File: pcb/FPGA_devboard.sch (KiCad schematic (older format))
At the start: 2 parts, among them X5 Conn_02x06_Odd_Even, X6 AC7020

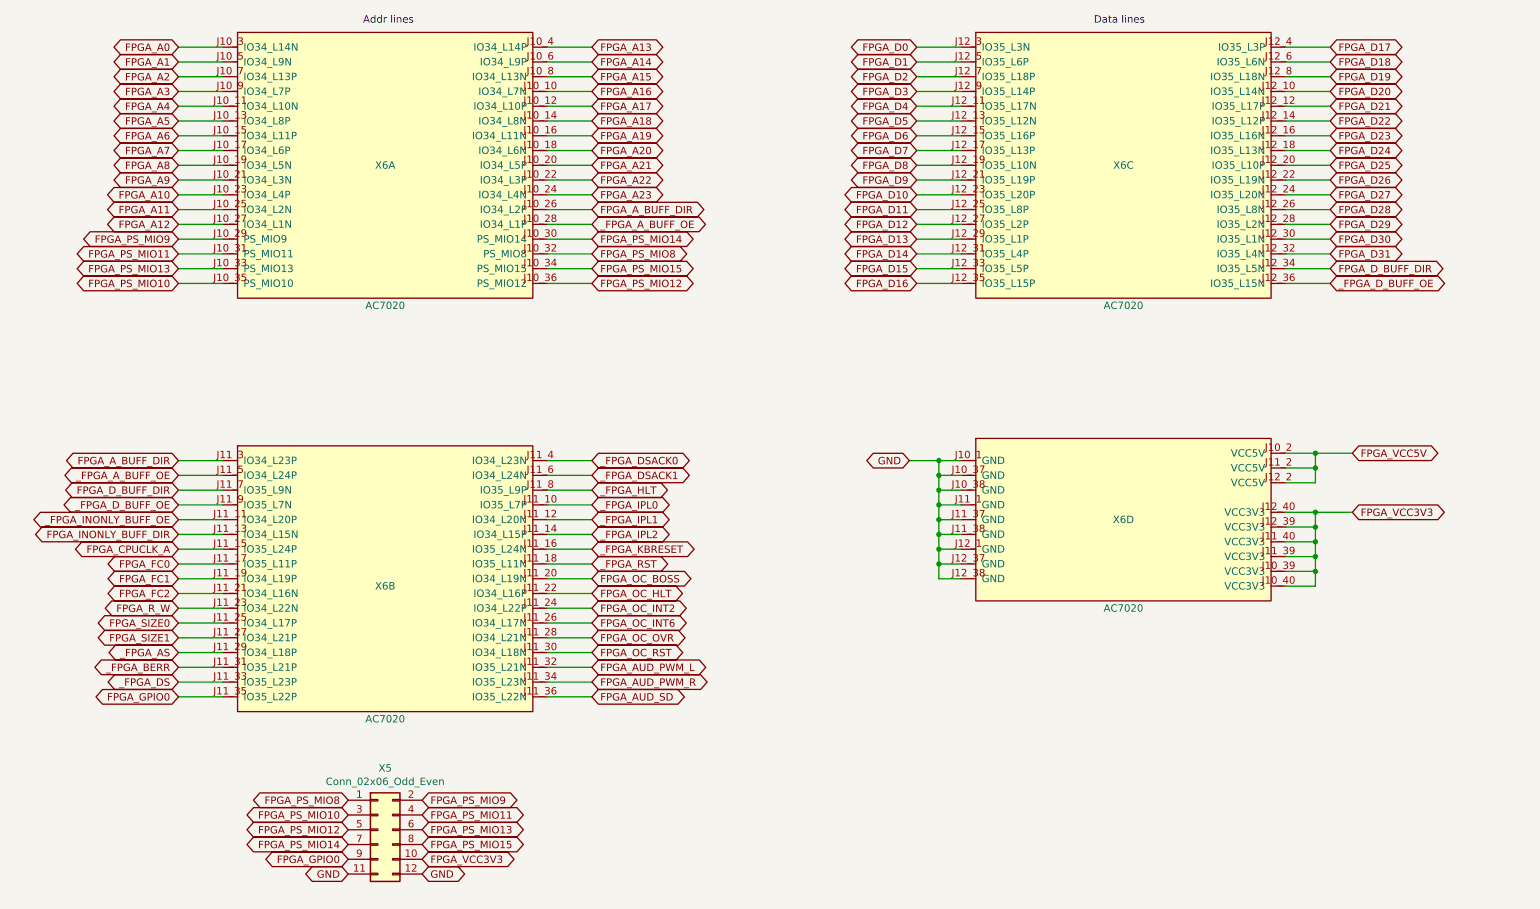
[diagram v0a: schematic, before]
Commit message: Some more changes wip
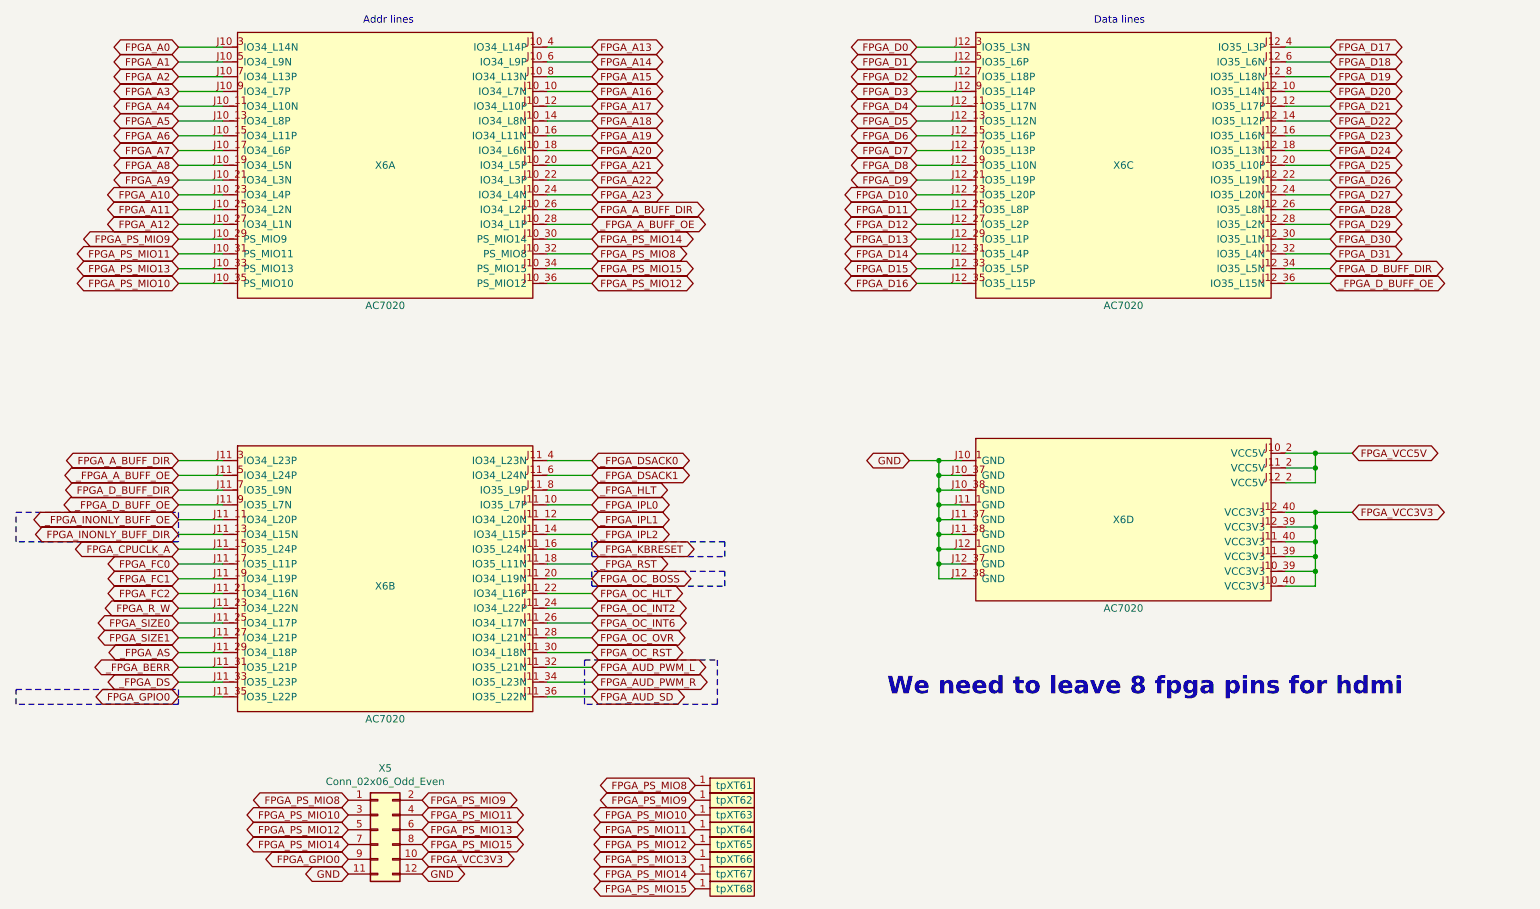
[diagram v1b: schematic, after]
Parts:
- added XT61, XT62, XT63, XT64, XT65, XT66, XT67, XT68: testpoint, symbol WM1200:testpoint
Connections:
- net FPGA_PS_MIO10: now also XT63.1 (tp)
- net FPGA_PS_MIO11: now also XT64.1 (tp)
- net FPGA_PS_MIO12: now also XT65.1 (tp)
- net FPGA_PS_MIO13: now also XT66.1 (tp)
- net FPGA_PS_MIO14: now also XT67.1 (tp)
- net FPGA_PS_MIO15: now also XT68.1 (tp)
- net FPGA_PS_MIO8: now also XT61.1 (tp)
- net FPGA_PS_MIO9: now also XT62.1 (tp)
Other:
- note added: "We need to leave 8 fpga pins for hdmi"
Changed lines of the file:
@@
 Wire Wire Line
 	4600 3200 4300 3200
+$Comp
+L WM1200:testpoint XT61
+U 1 1 5E5A11BD
+P 5550 6650
+F 0 "XT61" H 5600 6700 50  0000 C CNN
+F 1 "testpoint" H 5550 6800 50  0001 C CNN
+F 2 "" H 5550 6650 50  0001 C CNN
+F 3 "" H 5550 6650 50  0001 C CNN
+	1    5550 6650
+	1    0    0    -1
+$EndComp
+$Comp
+L WM1200:testpoint XT62
+U 1 1 5E5B690A
+P 5550 6750
+F 0 "XT62" H 5600 6800 50  0000 C CNN
+F 1 "testpoint" H 5550 6900 50  0001 C CNN
+F 2 "" H 5550 6750 50  0001 C CNN
+F 3 "" H 5550 6750 50  0001 C CNN
+	1    5550 6750
+	1    0    0    -1
+$EndComp
+$Comp
+L WM1200:testpoint XT63
+U 1 1 5E5BE856
+P 5550 6850
+F 0 "XT63" H 5600 6900 50  0000 C CNN
+F 1 "testpoint" H 5550 7000 50  0001 C CNN
+F 2 "" H 5550 6850 50  0001 C CNN
+F 3 "" H 5550 6850 50  0001 C CNN
+	1    5550 6850
+	1    0    0    -1
+$EndComp
+$Comp
+L WM1200:testpoint XT64
+U 1 1 5E5C67D2
+P 5550 6950
+F 0 "XT64" H 5600 7000 50  0000 C CNN
+F 1 "testpoint" H 5550 7100 50  0001 C CNN
+F 2 "" H 5550 6950 50  0001 C CNN
+F 3 "" H 5550 6950 50  0001 C CNN
+	1    5550 6950
+	1    0    0    -1
+$EndComp
+$Comp
+L WM1200:testpoint XT65
+U 1 1 5E5CE745
+P 5550 7050
+F 0 "XT65" H 5600 7100 50  0000 C CNN
+F 1 "testpoint" H 5550 7200 50  0001 C CNN
+F 2 "" H 5550 7050 50  0001 C CNN
+F 3 "" H 5550 7050 50  0001 C CNN
+	1    5550 7050
+	1    0    0    -1
+$EndComp
+$Comp
+L WM1200:testpoint XT66
+U 1 1 5E5D6657
+P 5550 7150
+F 0 "XT66" H 5600 7200 50  0000 C CNN
+F 1 "testpoint" H 5550 7300 50  0001 C CNN
+F 2 "" H 5550 7150 50  0001 C CNN
+F 3 "" H 5550 7150 50  0001 C CNN
+	1    5550 7150
+	1    0    0    -1
+$EndComp
+$Comp
+L WM1200:testpoint XT67
+U 1 1 5E5DE64C
+P 5550 7250
+F 0 "XT67" H 5600 7300 50  0000 C CNN
+F 1 "testpoint" H 5550 7400 50  0001 C CNN
+F 2 "" H 5550 7250 50  0001 C CNN
+F 3 "" H 5550 7250 50  0001 C CNN
+	1    5550 7250
+	1    0    0    -1
+$EndComp
+$Comp
+L WM1200:testpoint XT68
+U 1 1 5E5E66B0
+P 5550 7350
+F 0 "XT68" H 5600 7400 50  0000 C CNN
+F 1 "testpoint" H 5550 7500 50  0001 C CNN
+F 2 "" H 5550 7350 50  0001 C CNN
+F 3 "" H 5550 7350 50  0001 C CNN
+	1    5550 7350
+	1    0    0    -1
+$EndComp
+Text GLabel 5300 6600 0    50   BiDi ~ 0
+FPGA_PS_MIO8
+Text GLabel 5300 6700 0    50   BiDi ~ 0
+FPGA_PS_MIO9
+Text GLabel 5300 6800 0    50   BiDi ~ 0
+FPGA_PS_MIO10
+Text GLabel 5300 6900 0    50   BiDi ~ 0
+FPGA_PS_MIO11
+Text GLabel 5300 7000 0    50   BiDi ~ 0
+FPGA_PS_MIO12
+Text GLabel 5300 7100 0    50   BiDi ~ 0
+FPGA_PS_MIO13
+Text GLabel 5300 7200 0    50   BiDi ~ 0
+FPGA_PS_MIO14
+Text GLabel 5300 7300 0    50   BiDi ~ 0
+FPGA_PS_MIO15
+Text Notes 6600 6000 0    118  ~ 24
+We need to leave 8 fpga pins for hdmi
+Wire Notes Line
+	5450 5750 5450 6050
+Wire Notes Line
+	5450 6050 4550 6050
+Wire Notes Line
+	4550 6050 4550 5750
+Wire Notes Line
+	4550 5750 5450 5750
+Wire Notes Line
+	5500 5150 4600 5150
+Wire Notes Line
+	4600 5150 4600 5250
+Wire Notes Line
+	4600 5250 5500 5250
+Wire Notes Line
+	5500 5250 5500 5150
+Wire Notes Line
+	700  4750 1800 4750
+Wire Notes Line
+	1800 4750 1800 4950
+Wire Notes Line
+	1800 4950 700  4950
+Wire Notes Line
+	700  4950 700  4750
+Wire Notes Line
+	4600 4950 4600 5050
+Wire Notes Line
+	4600 5050 5500 5050
+Wire Notes Line
+	5500 5050 5500 4950
+Wire Notes Line
+	5500 4950 4600 4950
+Wire Notes Line
+	1800 5950 1800 6050
+Wire Notes Line
+	1800 6050 700  6050
+Wire Notes Line
+	700  6050 700  5950
+Wire Notes Line
+	700  5950 1800 5950
 $EndSCHEMATC

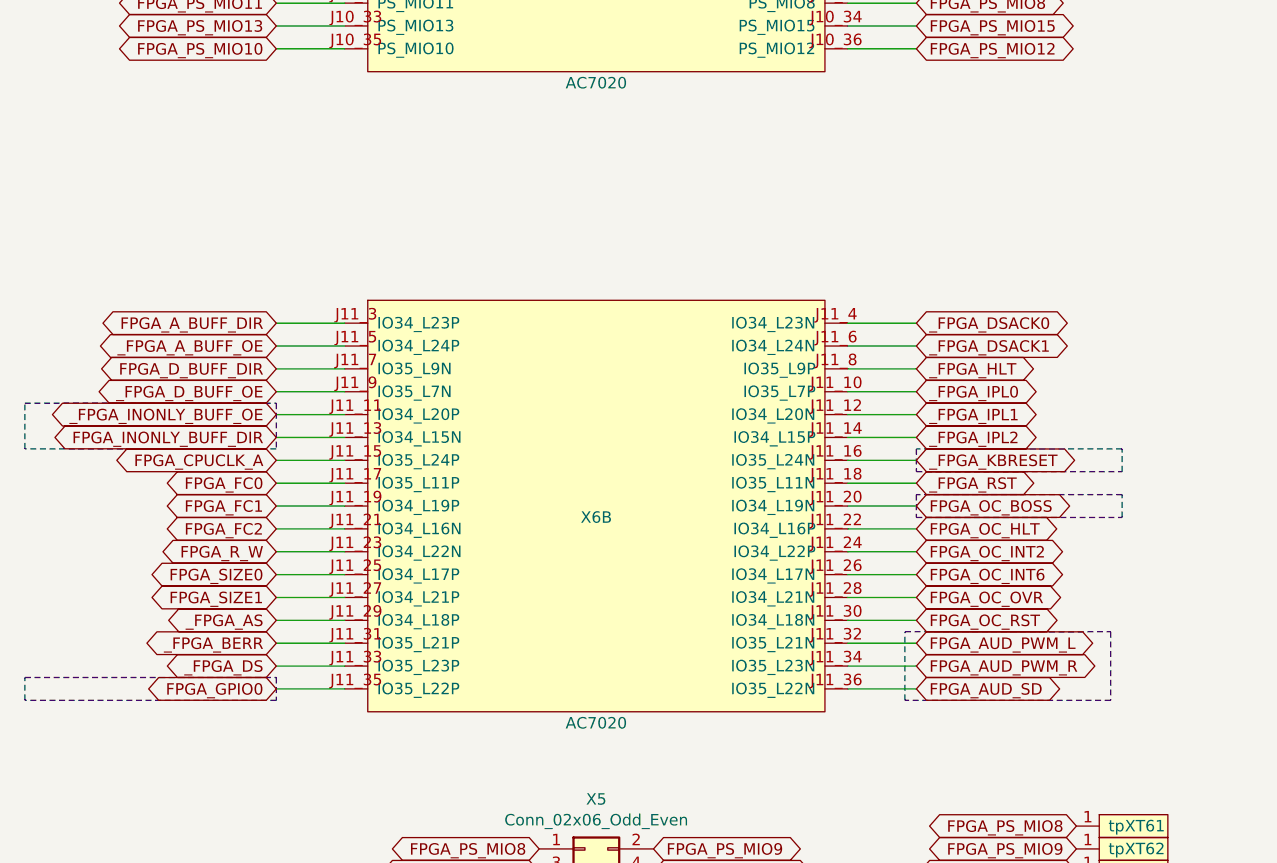
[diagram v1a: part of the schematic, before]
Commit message: hdmi list added
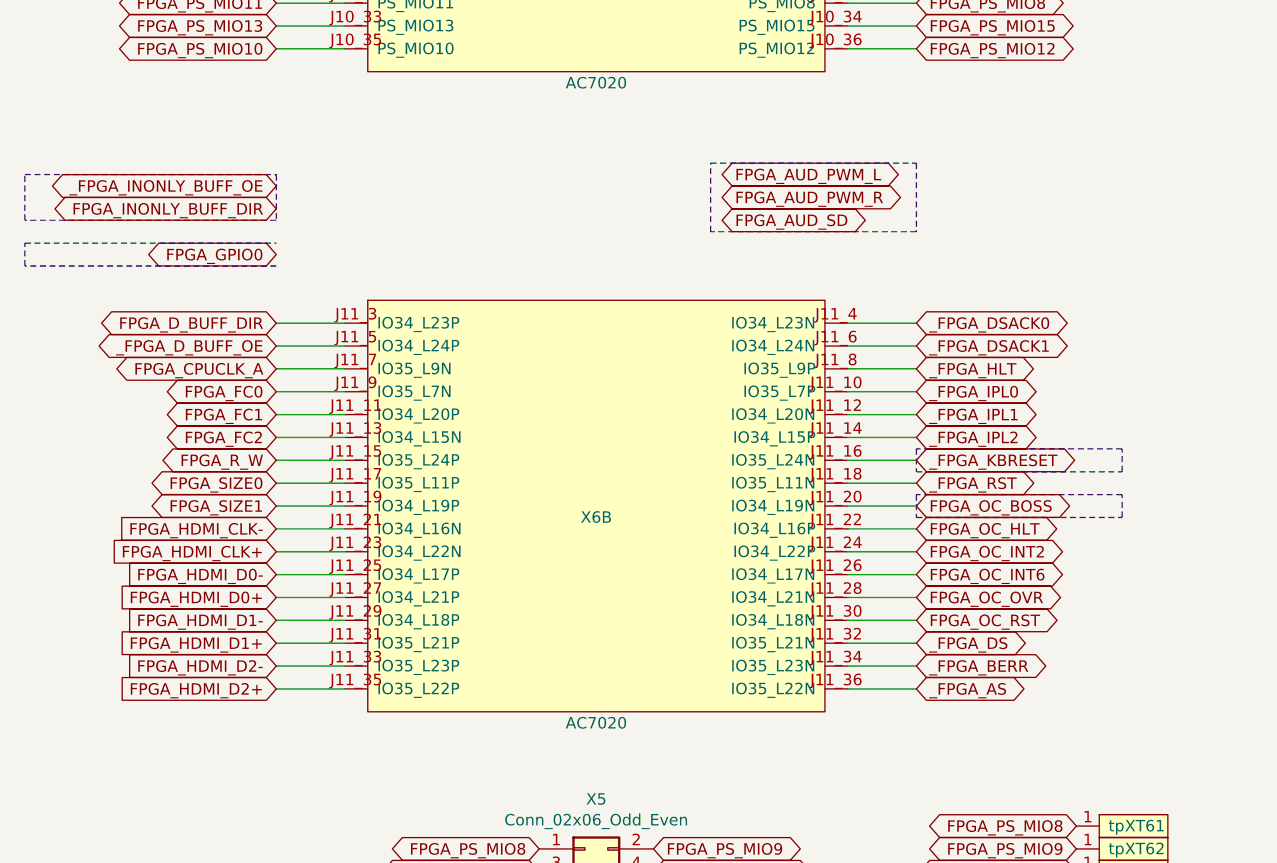
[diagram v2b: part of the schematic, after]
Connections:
- net FPGA_AUD_PWM_L: no longer X6.J11_32 (IO35_L21N)
- net FPGA_AUD_PWM_R: no longer X6.J11_34 (IO35_L23N)
- net FPGA_AUD_SD: no longer X6.J11_36 (IO35_L22N)
- net FPGA_A_BUFF_DIR: no longer X6.J11_3 (IO34_L23P)
- net FPGA_CPUCLK_A: now also X6.J11_7 (IO35_L9N); no longer X6.J11_15 (IO35_L24P)
- net FPGA_D_BUFF_DIR: now also X6.J11_3 (IO34_L23P); no longer X6.J11_7 (IO35_L9N)
- net FPGA_FC0: now also X6.J11_9 (IO35_L7N); no longer X6.J11_17 (IO35_L11P)
- net FPGA_FC1: now also X6.J11_11 (IO34_L20P); no longer X6.J11_19 (IO34_L19P)
- net FPGA_FC2: now also X6.J11_13 (IO34_L15N); no longer X6.J11_21 (IO34_L16N)
- net FPGA_GPIO0: no longer X6.J11_35 (IO35_L22P)
- net FPGA_INONLY_BUFF_DIR: no longer X6.J11_13 (IO34_L15N)
- net FPGA_R_W: now also X6.J11_15 (IO35_L24P); no longer X6.J11_23 (IO34_L22N)
- net FPGA_SIZE0: now also X6.J11_17 (IO35_L11P); no longer X6.J11_25 (IO34_L17P)
- net FPGA_SIZE1: now also X6.J11_19 (IO34_L19P); no longer X6.J11_27 (IO34_L21P)
- net _FPGA_AS: now also X6.J11_36 (IO35_L22N); no longer X6.J11_29 (IO34_L18P)
- net _FPGA_A_BUFF_OE: no longer X6.J11_5 (IO34_L24P)
- net _FPGA_BERR: now also X6.J11_34 (IO35_L23N); no longer X6.J11_31 (IO35_L21P)
- net _FPGA_DS: now also X6.J11_32 (IO35_L21N); no longer X6.J11_33 (IO35_L23P)
- net _FPGA_D_BUFF_OE: now also X6.J11_5 (IO34_L24P); no longer X6.J11_9 (IO35_L7N)
- net _FPGA_INONLY_BUFF_OE: no longer X6.J11_11 (IO34_L20P)
- new net FPGA_HDMI_CLK+: X6.J11_23 (IO34_L22N)
- new net FPGA_HDMI_CLK-: X6.J11_21 (IO34_L16N)
- new net FPGA_HDMI_D0+: X6.J11_27 (IO34_L21P)
- new net FPGA_HDMI_D0-: X6.J11_25 (IO34_L17P)
- new net FPGA_HDMI_D1+: X6.J11_31 (IO35_L21P)
- new net FPGA_HDMI_D1-: X6.J11_29 (IO34_L18P)
- new net FPGA_HDMI_D2+: X6.J11_35 (IO35_L22P)
- new net FPGA_HDMI_D2-: X6.J11_33 (IO35_L23P)
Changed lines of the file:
@@
 $Descr A4 11693 8268
 encoding utf-8
-Sheet 11 11
+Sheet 11 12
 Title "WishMaster 1200"
 Date ""
@@
 Text GLabel 9600 3200 2    50   BiDi ~ 0
 _FPGA_D_BUFF_OE
-Text GLabel 4600 5800 2    50   BiDi ~ 0
+Text GLabel 3750 3750 2    50   BiDi ~ 0
 FPGA_AUD_PWM_L
-Text GLabel 4600 5900 2    50   BiDi ~ 0
+Text GLabel 3750 3850 2    50   BiDi ~ 0
 FPGA_AUD_PWM_R
-Text GLabel 4600 6000 2    50   BiDi ~ 0
+Text GLabel 3750 3950 2    50   BiDi ~ 0
 FPGA_AUD_SD
-Text GLabel 1800 4400 0    50   BiDi ~ 0
-FPGA_A_BUFF_DIR
-Text GLabel 1800 4700 0    50   BiDi ~ 0
-_FPGA_D_BUFF_OE
-Text GLabel 1800 4500 0    50   BiDi ~ 0
-_FPGA_A_BUFF_OE
-Text GLabel 1800 4600 0    50   BiDi ~ 0
-FPGA_D_BUFF_DIR
-Text GLabel 1800 4800 0    50   BiDi ~ 0
-_FPGA_INONLY_BUFF_OE
-Text GLabel 1800 4900 0    50   BiDi ~ 0
-FPGA_INONLY_BUFF_DIR
-Text GLabel 1800 5000 0    50   BiDi ~ 0
-FPGA_CPUCLK_A
-Text GLabel 1800 5100 0    50   BiDi ~ 0
-FPGA_FC0
-Text GLabel 1800 5200 0    50   BiDi ~ 0
-FPGA_FC1
-Text GLabel 1800 5300 0    50   BiDi ~ 0
-FPGA_FC2
 Text GLabel 4600 5200 2    50   BiDi ~ 0
 FPGA_OC_BOSS
@@
 Text GLabel 4600 5700 2    50   BiDi ~ 0
 FPGA_OC_RST
-Text GLabel 1800 5400 0    50   BiDi ~ 0
-FPGA_R_W
-Text GLabel 1800 5500 0    50   BiDi ~ 0
-FPGA_SIZE0
-Text GLabel 1800 5600 0    50   BiDi ~ 0
-FPGA_SIZE1
-Text GLabel 1800 5700 0    50   BiDi ~ 0
-_FPGA_AS
-Text GLabel 1800 5800 0    50   BiDi ~ 0
-_FPGA_BERR
-Text GLabel 1800 5900 0    50   BiDi ~ 0
-_FPGA_DS
 Text GLabel 4600 4400 2    50   BiDi ~ 0
 _FPGA_DSACK0
@@
 Text GLabel 3450 7100 2    50   BiDi ~ 0
 FPGA_VCC3V3
-Text GLabel 1800 6000 0    50   BiDi ~ 0
+Text GLabel 1800 4100 0    50   BiDi ~ 0
 FPGA_GPIO0
 Text GLabel 2950 7100 0    50   BiDi ~ 0
@@
 We need to leave 8 fpga pins for hdmi
 Wire Notes Line
-	5450 5750 5450 6050
-Wire Notes Line
-	5450 6050 4550 6050
-Wire Notes Line
-	4550 6050 4550 5750
-Wire Notes Line
-	4550 5750 5450 5750
+	4600 3700 4600 4000
+Wire Notes Line
+	4600 4000 3700 4000
+Wire Notes Line
+	3700 3700 4600 3700
 Wire Notes Line
 	5500 5150 4600 5150
@@
 	5500 5250 5500 5150
 Wire Notes Line
-	700  4750 1800 4750
-Wire Notes Line
-	1800 4750 1800 4950
-Wire Notes Line
-	1800 4950 700  4950
-Wire Notes Line
-	700  4950 700  4750
+	1800 3750 1800 3950
+Wire Notes Line
+	700  3950 700  3750
 Wire Notes Line
 	4600 4950 4600 5050
@@
 	5500 4950 4600 4950
 Wire Notes Line
-	1800 5950 1800 6050
-Wire Notes Line
-	1800 6050 700  6050
-Wire Notes Line
-	700  6050 700  5950
-Wire Notes Line
-	700  5950 1800 5950
+	1800 4150 700  4150
+Wire Notes Line
+	700  4150 700  4050
+Wire Notes Line
+	700  4050 1800 4050
+Text GLabel 1800 6000 0    50   Input ~ 0
+FPGA_HDMI_D2+
+Text GLabel 1800 5900 0    50   Input ~ 0
+FPGA_HDMI_D2-
+Text GLabel 1800 5800 0    50   Input ~ 0
+FPGA_HDMI_D1+
+Text GLabel 1800 5600 0    50   Input ~ 0
+FPGA_HDMI_D0+
+Text GLabel 1800 5500 0    50   Input ~ 0
+FPGA_HDMI_D0-
+Text GLabel 1800 5700 0    50   Input ~ 0
+FPGA_HDMI_D1-
+Text GLabel 1800 5400 0    50   Input ~ 0
+FPGA_HDMI_CLK+
+Text GLabel 1800 5300 0    50   Input ~ 0
+FPGA_HDMI_CLK-
+Wire Notes Line
+	1800 3950 700  3950
+Wire Notes Line
+	700  3750 1800 3750
+Text GLabel 4600 5800 2    50   BiDi ~ 0
+_FPGA_DS
+Text GLabel 4600 5900 2    50   BiDi ~ 0
+_FPGA_BERR
+Text GLabel 4600 6000 2    50   BiDi ~ 0
+_FPGA_AS
+Text GLabel 1800 5200 0    50   BiDi ~ 0
+FPGA_SIZE1
+Text GLabel 1800 5100 0    50   BiDi ~ 0
+FPGA_SIZE0
+Text GLabel 1800 5000 0    50   BiDi ~ 0
+FPGA_R_W
+Text GLabel 1800 4900 0    50   BiDi ~ 0
+FPGA_FC2
+Text GLabel 1800 4800 0    50   BiDi ~ 0
+FPGA_FC1
+Text GLabel 1800 4700 0    50   BiDi ~ 0
+FPGA_FC0
+Text GLabel 1800 4600 0    50   BiDi ~ 0
+FPGA_CPUCLK_A
+Text GLabel 1800 3900 0    50   BiDi ~ 0
+FPGA_INONLY_BUFF_DIR
+Text GLabel 1800 3800 0    50   BiDi ~ 0
+_FPGA_INONLY_BUFF_OE
+Text GLabel 1800 4400 0    50   BiDi ~ 0
+FPGA_D_BUFF_DIR
+Text GLabel 1800 4500 0    50   BiDi ~ 0
+_FPGA_D_BUFF_OE
+Wire Notes Line
+	3700 4000 3700 3700
 $EndSCHEMATC
